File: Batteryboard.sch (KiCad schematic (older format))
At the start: 95 parts, among them J1 Conn_01x02_Male, J2 Conn_01x03_Male, J3 Conn_01x02_Male, J4 Conn_01x02_Male, J5 SC_19-20, Q1 SI7617DN-T1-GE3, Q2 SI7617DN-T1-GE3, Q3 SI7617DN-T1-GE3, Q4 SIS412DN-T1-GE3, Q5 SIS412DN-T1-GE3, Q6 SIS412DN-T1-GE3, Q7 SI7617DN-T1-GE3, Q8 SIS412DN-T1-GE3, Q9 SIS412DN-T1-GE3, SW1 SW_DIP_x01, U1 BQ24617RGET, U2 TPS65279DAPR, U3 BQ29200DRBT

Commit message: made lots of progress schematic wise, still need to add a few things to be sure, but its progress
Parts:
- removed J3: Conn_01x02_Male, Connector_TE-Connectivity:TE_MATE-N-LOK_1-770866-x_1x02_P4.14mm_Vertical, symbol Connector:Conn_01x02_Male
- removed Q9: SIS412DN-T1-GE3, SI7617DN-T1-GE3:SIS862DNT1GE3, symbol Batteryboard-rescue:SI7617DN-T1-GE3-SI7617DN-T1-GE3
- removed R10: 10kOhm, Resistor_SMD:R_0805_2012Metric, symbol Device:R_US
- removed R9: 27kOhm, Resistor_SMD:R_0805_2012Metric, symbol Device:R_US
- removed SW1: SW_DIP_x01, PololuSwitch:PololuSwitch, symbol Switch:SW_DIP_x01
- added C23, C44, C45, C46, C47, C48, C49: 22uF, Capacitor_SMD:C_0603_1608Metric, symbol Device:C
- added C24, C26, C27, C28, C29, C34, C35, C38: C, Capacitor_SMD:C_0603_1608Metric, symbol Device:C
- added C32, C40: 100nf, Capacitor_SMD:C_0603_1608Metric, symbol Device:C
- added C33, C39, C43: 1nf, Capacitor_SMD:C_0603_1608Metric, symbol Device:C
- added C36, C37, C41, C42: 100pf, Capacitor_SMD:C_0603_1608Metric, symbol Device:C
- added D5: D5V0L2B3W-7, Package_TO_SOT_SMD:SOT-23, symbol Device:D_TVS_x2_CAA
- added L2: 4.7uH, Inductor_SMD:L_Vishay_IHLP-2525, symbol Device:L
- added NP1, NP2: 120, Resistor_SMD:R_0603_1608Metric, symbol Device:R_US
- added R25, R26, R27, R28, R29, R32, R33: R_US, Resistor_SMD:R_0603_1608Metric, symbol Device:R_US
- added R34, R35, R37: 0, Resistor_SMD:R_0603_1608Metric, symbol Device:R_US
- added R36: 10k, Resistor_SMD:R_0603_1608Metric, symbol Device:R_US
- added U4: PIC18F25K50-I_SO, PIC18F25K50-ISO:PIC18F25K50-I&slash_SO, symbol PIC18F25K50-ISO:PIC18F25K50-I_SO
- added U5: MCP2515-xSO, Package_SO:SOIC-18W_7.5x11.6mm_P1.27mm, symbol Interface_CAN_LIN:MCP2515-xSO
- added U6: SN65HVD1050D, Package_SO:SOIC-8_3.9x4.9mm_P1.27mm, symbol Interface_CAN_LIN:SN65HVD1050D
- C17, C18, C19, C20, C21, C22: footprint (none) -> Capacitor_SMD:C_0603_1608Metric
- C25, C30: renamed from C?; footprint (none) -> Capacitor_SMD:C_0603_1608Metric
- C31: renamed from C?; value 22uF x 4 -> 22uF; footprint (none) -> Capacitor_SMD:C_0603_1608Metric
- CTTC1: footprint Capacitor_SMD:C_1206_3216Metric -> Capacitor_SMD:C_0603_1608Metric
- D2, D3, D4: footprint Diode_THT:D_5KP_P7.62mm_Vertical_AnodeUp -> Diode_SMD:D_0603_1608Metric
- J2: footprint Connector_JST:JST_EH_B3B-EH-A_1x03_P2.50mm_Vertical -> Connector_JST:JST_XH_B3B-XH-AM_1x03_P2.50mm_Vertical
- L1: footprint Inductor_SMD:L_0603_1608Metric -> Inductor_SMD:L_Vishay_IHLP-2525
- L3: renamed from L?; footprint (none) -> Inductor_SMD:L_Vishay_IHLP-2525
- R1, R10/RT1, R11, R12, R13, R14, R15, R16, R17, R18, R19, R2, R20, R3, R4, R5, R6, R7, R8, R9/RT2, RAC1, RCB_EXT1, RCLAMP1, RIN1, RIN2, ROUT1, RSR1, RVD1: footprint Resistor_SMD:R_0805_2012Metric -> Resistor_SMD:R_0603_1608Metric
- R21, R22, R23, R24: footprint (none) -> Resistor_SMD:R_0603_1608Metric
- R30, R31: renamed from R?; footprint (none) -> Resistor_SMD:R_0603_1608Metric
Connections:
- net labels added: CS, INT, MCLR, RESET, RX0BF, RX1BF, SCK, SI, SO, TEMP_OUT, TX0RTS, TX1RTS, TX2RTS, VDD, VSS
- net labels removed: FB2
- wire segments 380 -> 441
- no-connect marks 0 -> 3
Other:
- moved on the sheet: C1, C10, C11, C12, C13, C14, C15, C16, C17, C18, C19, C2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

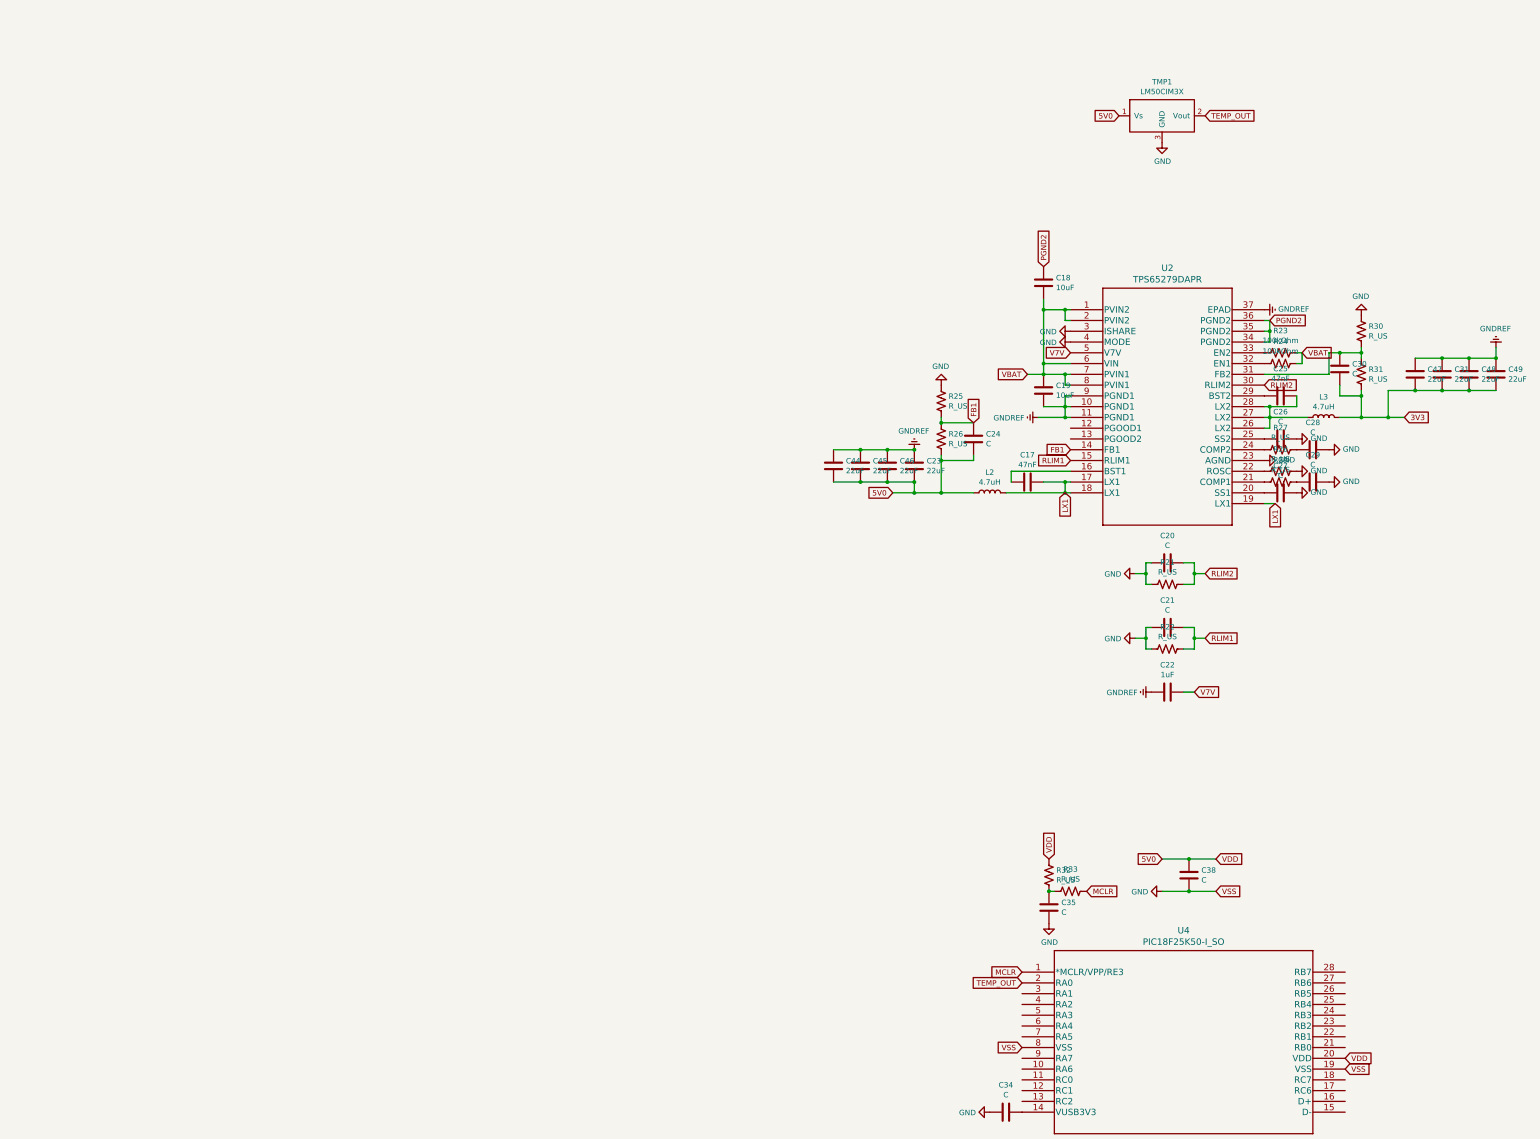
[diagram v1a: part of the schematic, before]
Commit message: more progress on the way to being done, added a bunch of stuff having to do with current sense
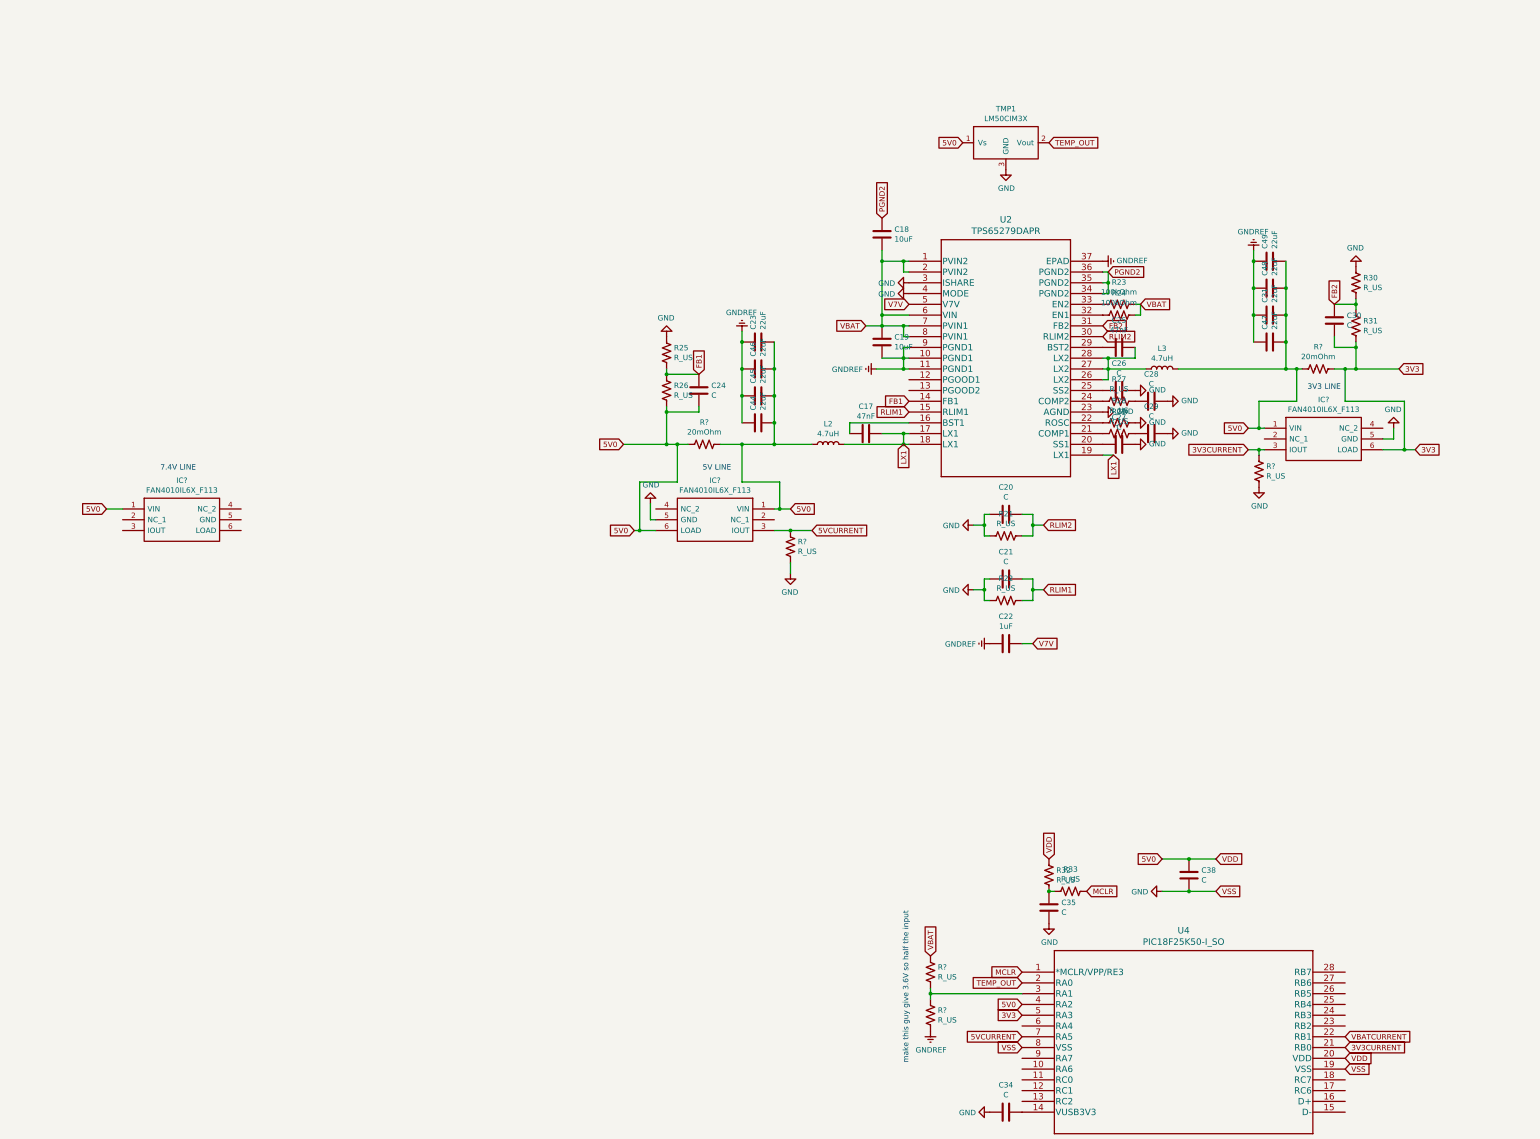
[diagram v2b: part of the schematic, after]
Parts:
- added IC? (x3): FAN4010IL6X_F113, 6-LEAD_MICROPAK, symbol FAN4010IL6X_F113:FAN4010IL6X_F113
- added R? (x4): R_US, symbol Device:R_US
- added R? (x2): 20mOhm, symbol Device:R_US
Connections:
- net 3V3: now also U4.5 (RA3), IC?.6 (LOAD), R?.1; no longer C31.2, C47.2, C48.2, C49.2, L3.2
- net 5V0: now also C31.2, C47.2, C48.2, C49.2, L3.2, U4.4 (RA2), IC?.1 (VIN), IC?.1 (VIN), IC?.1 (VIN), IC?.6 (LOAD), R?.1, R?.2, R?.2
- net GND: now also IC?.5 (GND), IC?.5 (GND), R?.2, R?.2, R?.2
- net Q4D: now also R?.1
- net FB2: now reaches C30.1, R30.2, R31.1, U2.31 (FB2)
- net 3V3CURRENT: now reaches U4.21 (RB0)
- net 3V3CURRENT: now also IC?.3 (IOUT), R?.1
- net VBATCURRENT: now reaches U4.22 (RB1)
- net at U4.3 (RA1): now also R?.1, R?.2
- net 5VCURRENT: now reaches U4.7 (RA5)
- net 5VCURRENT: now also IC?.3 (IOUT), R?.1
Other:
- note added: "3V3 LINE"
- note added: "5V LINE"
- note added: "7.4V LINE"
- note added: "make this guy give 3.6V so half the input"
- moved on the sheet: C17, C18, C19, C20, C21, C22, C23, C24, C25, C26, C27, C28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

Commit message: finished schematic, more or less
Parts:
- added R38: R_US, Resistor_SMD:R_0603_1608Metric, symbol Device:R_US
- added R39: 20mOhm, Resistor_SMD:R_0603_1608Metric, symbol Device:R_US
- IC1, IC2, IC3: renamed from IC?; footprint 6-LEAD_MICROPAK -> FAN4010IL6X_F113:6-LEAD_MICROPAK
- J5: footprint MASA-LIB:Stack_Connector_2019_2020 -> MASA-LIB:bottom_Stack_Connector_2019_2020
- R10, R40, R41, R42, R43, R9: renamed from R?; footprint (none) -> Resistor_SMD:R_0603_1608Metric
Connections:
- net GBAT is gone; now on net GND: J4.1 (Pin_1)
- net 3V3CURRENT: now also U4.25 (RB4); no longer U4.21 (RB0)
- net 5V0: now also C15.1, C3.1, C8.1, C9.1, Q3.5 (D_1), Q3.6 (D_2), Q3.7 (D_3), Q3.8 (D_4), Q4.5 (D_1), Q4.6 (D_2), Q4.7 (D_3), Q4.8 (D_4), R15.1, RAC1.1, U1.1 (ACN), R39.2
- net CS: now also U4.18 (RC7)
- net GND: now also IC1.5 (GND), R38.1
- net INT: now also U4.23 (RB2)
- net RESET: now also U4.6 (RA4)
- net RX0BF: now also U4.10 (RA6)
- net RX1BF: now also U4.9 (RA7)
- net SCK: now also U4.22 (RB1)
- net SI: now also U4.24 (RB3)
- net SO: now also U4.21 (RB0)
- net TX0RTS: now also U4.13 (RC2)
- net TX1RTS: now also U4.12 (RC1)
- net TX2RTS: now also U4.11 (RC0)
- net VBATCURRENT: now also IC1.3 (IOUT), U4.26 (RB5), R38.2; no longer U4.22 (RB1)
- net TS: now reaches C1.2, R16.1, U1.6 (TS)
- net TS: now also U4.17 (RC6)
- net VBAT: now reaches IC1.6 (LOAD)
- net VBAT: now also C18.2, C19.1, R23.1, R24.1, R9.1, U2.1 (PVIN2), U2.2 (PVIN2), U2.6 (VIN), U2.7 (PVIN1), U2.8 (PVIN1), R39.1
- net at C37.2, R35.1: now also U6.1 (TXD); no longer U6.4 (RXD)
- net at R34.2: now also U6.4 (RXD); no longer U6.1 (TXD)
- removed net Q4D: C15.1, C18.2, C19.1, C3.1, C8.1, C9.1, Q3.5 (D_1), Q3.6 (D_2), Q3.7 (D_3), Q3.8 (D_4), Q4.5 (D_1), Q4.6 (D_2), Q4.7 (D_3), Q4.8 (D_4), R15.1, R23.1, R24.1, R9.1, RAC1.1, U1.1 (ACN), U2.1 (PVIN2), U2.2 (PVIN2), U2.6 (VIN), U2.7 (PVIN1), U2.8 (PVIN1)
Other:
- moved on the sheet: C1, C17, C18, C19, C20, C21, C22, C23, C24, C25, C26, C27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

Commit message: made progress on layout, charging IC is basically done
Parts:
- CTTC1: value 43nF -> 47nF
- J5: symbol MASA-LIB:SC_19-20 -> Batteryboard-rescue:SC_19-20-MASA-LIB
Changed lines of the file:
@@
 $EndComp
 $Comp
-L MASA-LIB:SC_19-20 J5
+L Batteryboard-rescue:SC_19-20-MASA-LIB J5
 U 1 1 5E021180
 P 1900 7150
@@
 P 3100 4350
 F 0 "CTTC1" H 3215 4396 50  0000 L CNN
-F 1 "43nF" H 3215 4305 50  0000 L CNN
+F 1 "47nF" H 3215 4305 50  0000 L CNN
 F 2 "Capacitor_SMD:C_0603_1608Metric" H 3100 4350 50  0001 C CNN
 F 3 "~" H 3100 4350 50  0001 C CNN
